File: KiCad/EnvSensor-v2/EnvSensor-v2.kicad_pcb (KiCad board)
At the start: 2 copper layers, 120 x 100 mm, 162 parts, among them J1 JTAG, J10 Conn_01x02, J2 Conn_01x02, J3 USB_B_Micro, J4 Conn_01x02, J5 Micro_SD_Card_Det, J6 Conn_01x02, J7 I2C, J8 HPMA115C0-003, J9 Conn_01x02, P1 USB_C_Plug_USB2.0, Q1 IRLML2502, Q2 Si3407DV, Q3 IRFR9024, Q4 AO6804A, SW1 SW_Push, SW2 Reset, SW3 SW_Push, SW4 SW_Push, SW5 SW_Push, SW6 Start, U1 STM32L451RCT6, U10 LTC3440, U11 MCP1826S-5.0, U12 MCP1825S-3.3, U13 ESP-12S, U2 E-Ink_Waveshare_4.2, U3 SCD30, U4 SCD40, U5 BMP280, U6 AP9101CK, U7 MCP73843-4.2, U8 BME280-Module, U9 LM2735XMF, Y1 16Hz, Y2 32768/12.5pF

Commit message: touchgfx introduced
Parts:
- Q3: value IRFR9024 -> ZXMP6A16K
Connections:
- net E_INK_CD renamed E_INK_DC

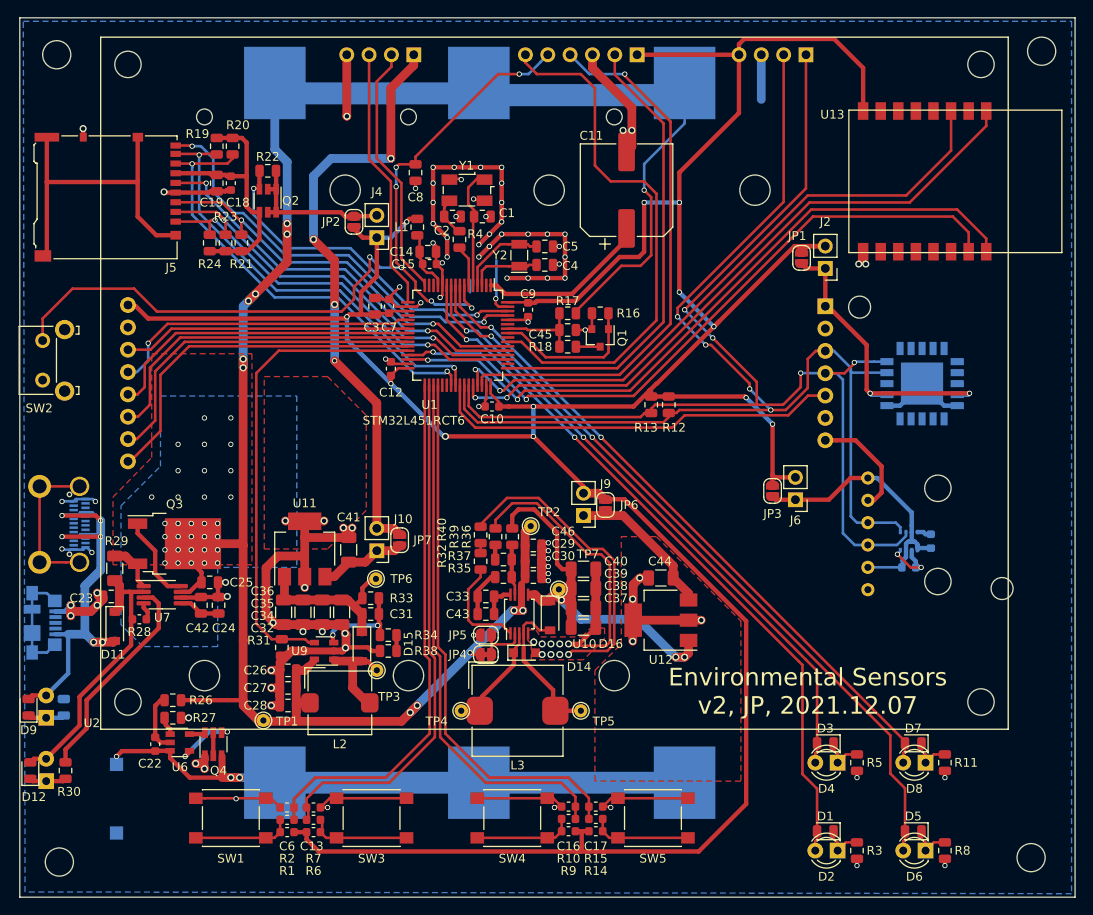
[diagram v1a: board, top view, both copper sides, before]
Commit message: More pcb work
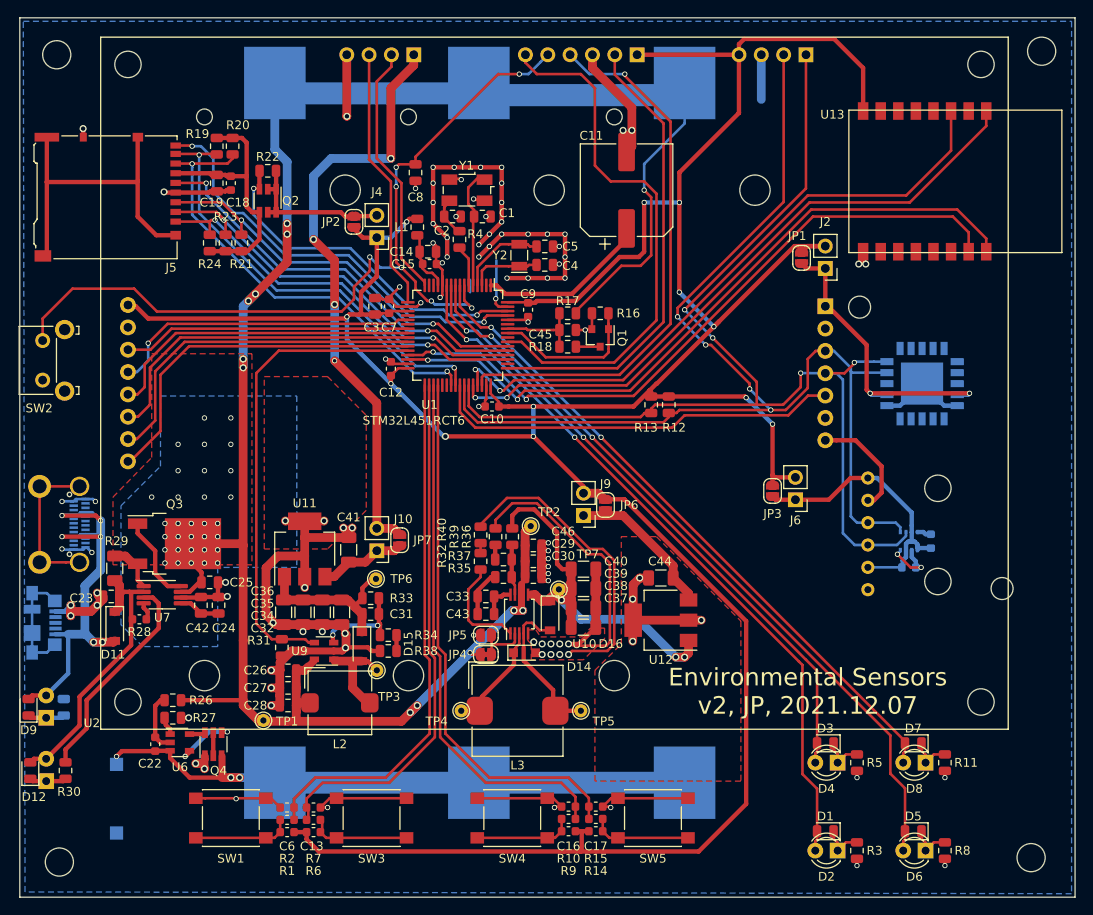
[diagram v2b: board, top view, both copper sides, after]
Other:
- net class Default removed
- net class Power removed
- net class Thick removed
